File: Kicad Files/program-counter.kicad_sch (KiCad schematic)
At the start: 7 parts, among them U23 74LS161, U24 74LS161, U25 74LS245

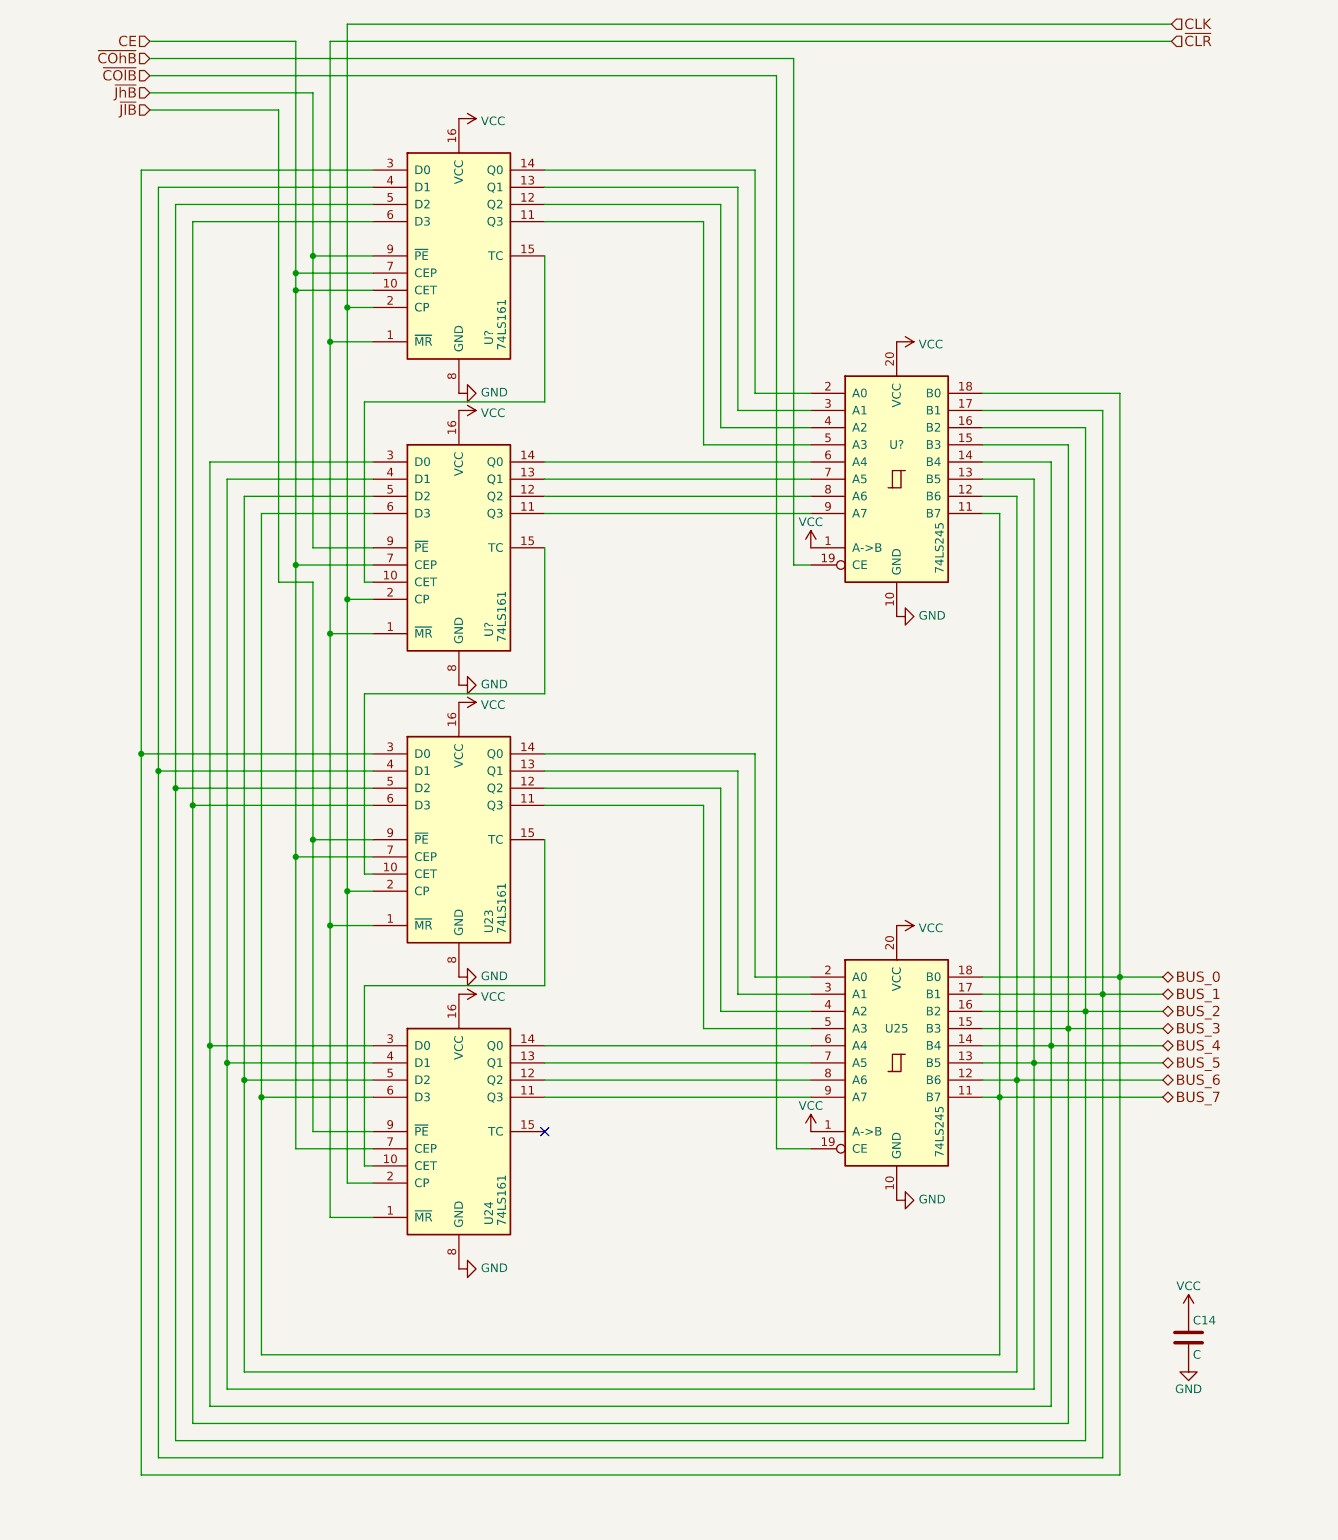
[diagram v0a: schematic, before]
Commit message: work on pc2
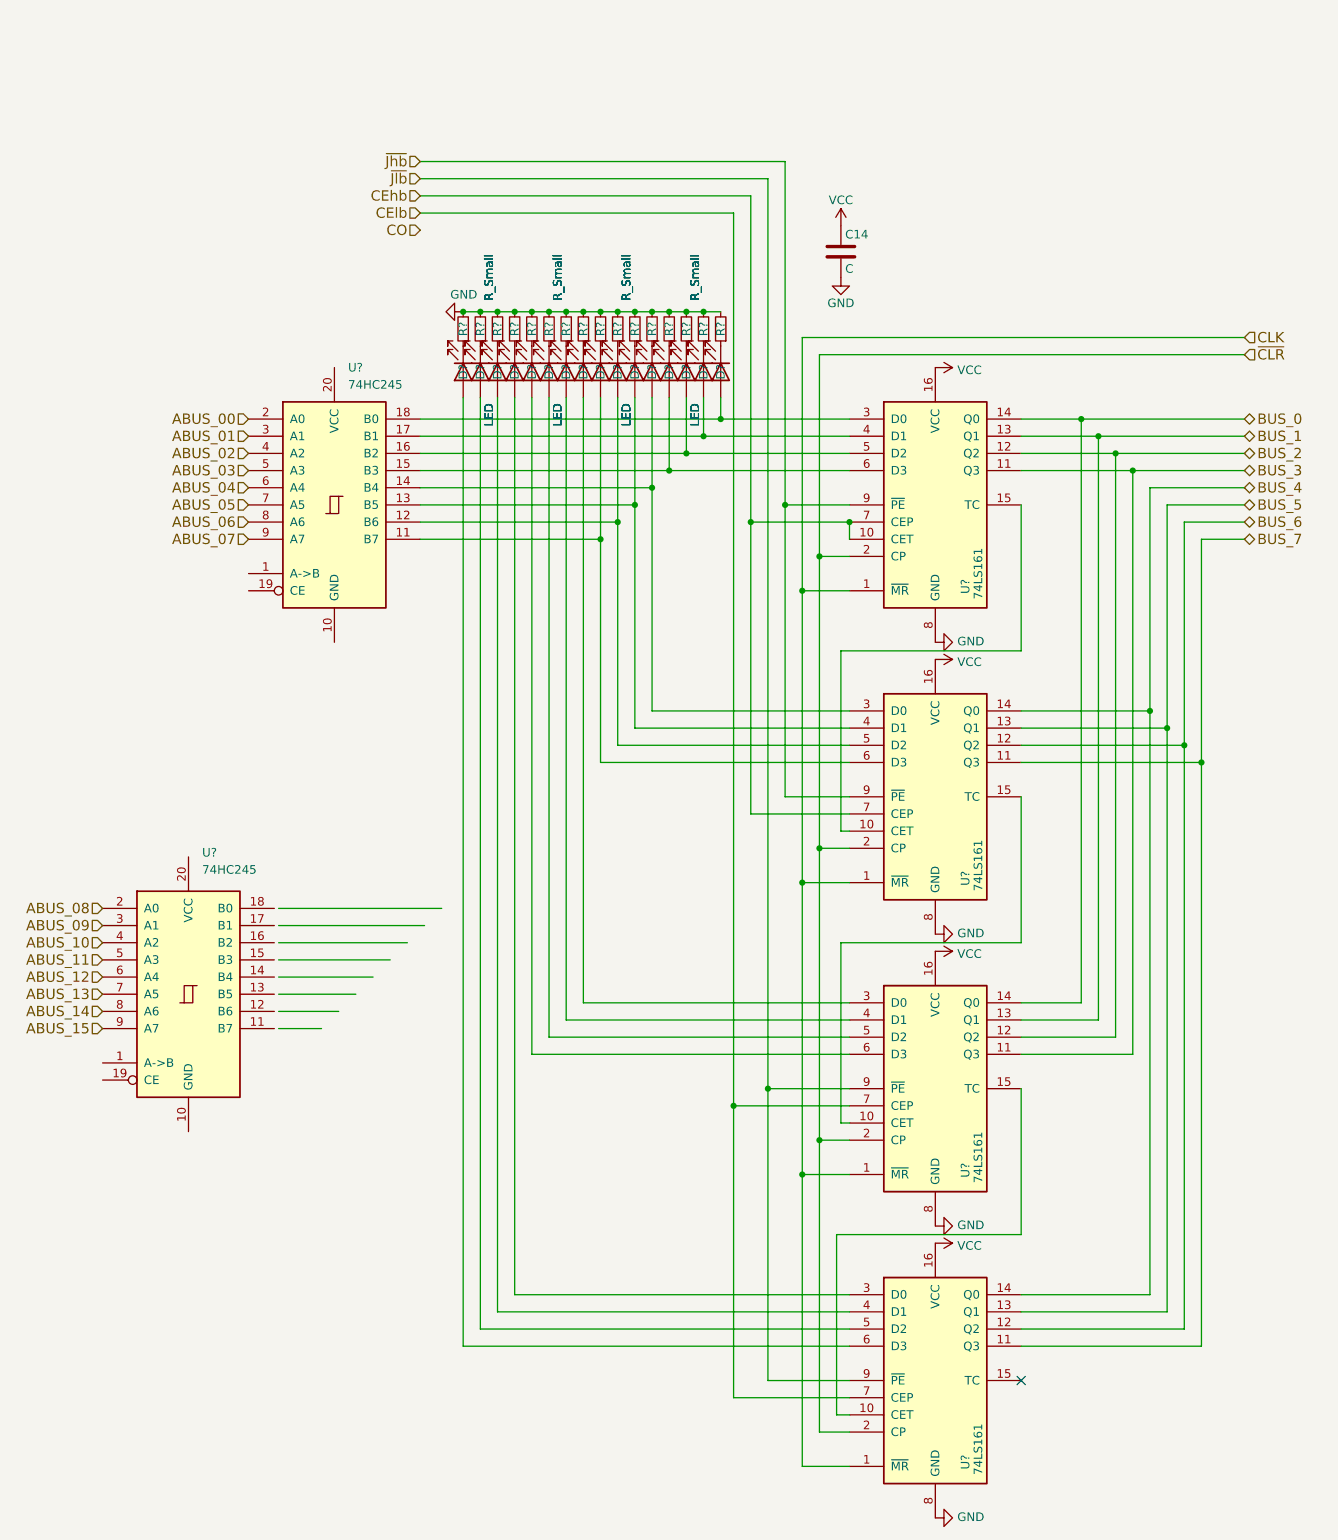
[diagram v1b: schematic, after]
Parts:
- removed U23, U24, U? (x2): 74LS161, symbol 74xx:74LS161
- removed U25, U?: 74LS245, symbol 74xx:74LS245
- added D? (x16): LED, symbol Device:LED
- added R? (x16): R_Small, symbol Device:R_Small
- added U? (x2): 74HC245, symbol 74xx:74HC245
- added U? (x4): 74LS161, symbol 74xx:74LS161
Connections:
- net BUS_0: now also U?.14 (Q0), U?.14 (Q0)
- net BUS_1: now also U?.13 (Q1), U?.13 (Q1)
- net BUS_2: now also U?.12 (Q2), U?.12 (Q2)
- net BUS_3: now also U?.11 (Q3), U?.11 (Q3)
- net BUS_4: now also U?.14 (Q0), U?.14 (Q0)
- net BUS_5: now also U?.13 (Q1), U?.13 (Q1)
- net BUS_6: now also U?.12 (Q2), U?.12 (Q2)
- net BUS_7: now also U?.11 (Q3), U?.11 (Q3)
- net CLK: now also U?.1 (~{MR}), U?.1 (~{MR}), U?.1 (~{MR}), U?.1 (~{MR})
- net GND: now also R?.2, R?.2, R?.2, R?.2, R?.2, R?.2, R?.2, R?.2, R?.2, R?.2, R?.2, R?.2, R?.2, R?.2, R?.2, R?.2, U?.8 (GND), U?.8 (GND), U?.8 (GND), U?.8 (GND)
- net VCC: now also U?.16 (VCC), U?.16 (VCC), U?.16 (VCC), U?.16 (VCC)
- net ~{CLR}: now also U?.2 (CP), U?.2 (CP), U?.2 (CP), U?.2 (CP)
- new net: D?.1 (K), R?.1 (x16)
- new net: D?.2 (A), U?.15 (B3), U?.6 (D3)
- new net: D?.2 (A), U?.5 (D2) (x2)
- new net: D?.2 (A), U?.18 (B0), U?.3 (D0)
- new net: D?.2 (A), U?.6 (D3) (x2)
- new net: D?.2 (A), U?.12 (B6), U?.5 (D2)
- new net: D?.2 (A), U?.3 (D0) (x2)
- new net: D?.2 (A), U?.17 (B1), U?.4 (D1)
- new net: U?.10 (CET), U?.15 (TC) (x3)
- new net: D?.2 (A), U?.4 (D1) (x2)
- new net: D?.2 (A), U?.14 (B4), U?.3 (D0)
- new net: D?.2 (A), U?.13 (B5), U?.4 (D1)
- new net: D?.2 (A), U?.11 (B7), U?.6 (D3)
- new net: D?.2 (A), U?.16 (B2), U?.5 (D2)
- new net ABUS_00: U?.2 (A0)
- new net ABUS_01: U?.3 (A1)
- new net ABUS_02: U?.4 (A2)
- new net ABUS_03: U?.5 (A3)
- new net ABUS_04: U?.6 (A4)
- new net ABUS_05: U?.7 (A5)
- new net ABUS_06: U?.8 (A6)
- new net ABUS_07: U?.9 (A7)
- new net ABUS_08: U?.2 (A0)
- new net ABUS_09: U?.3 (A1)
- new net ABUS_10: U?.4 (A2)
- new net ABUS_11: U?.5 (A3)
- new net ABUS_12: U?.6 (A4)
- new net ABUS_13: U?.7 (A5)
- new net ABUS_14: U?.8 (A6)
- new net ABUS_15: U?.9 (A7)
- new net CEhb: U?.10 (CET), U?.7 (CEP), U?.7 (CEP)
- new net CElb: U?.7 (CEP), U?.7 (CEP)
- new net ~{Jhb}: U?.9 (~{PE}), U?.9 (~{PE})
- new net ~{Jlb}: U?.9 (~{PE}), U?.9 (~{PE})
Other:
- moved on the sheet: C14
